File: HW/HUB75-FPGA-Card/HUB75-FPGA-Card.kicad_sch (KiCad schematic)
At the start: 4 parts

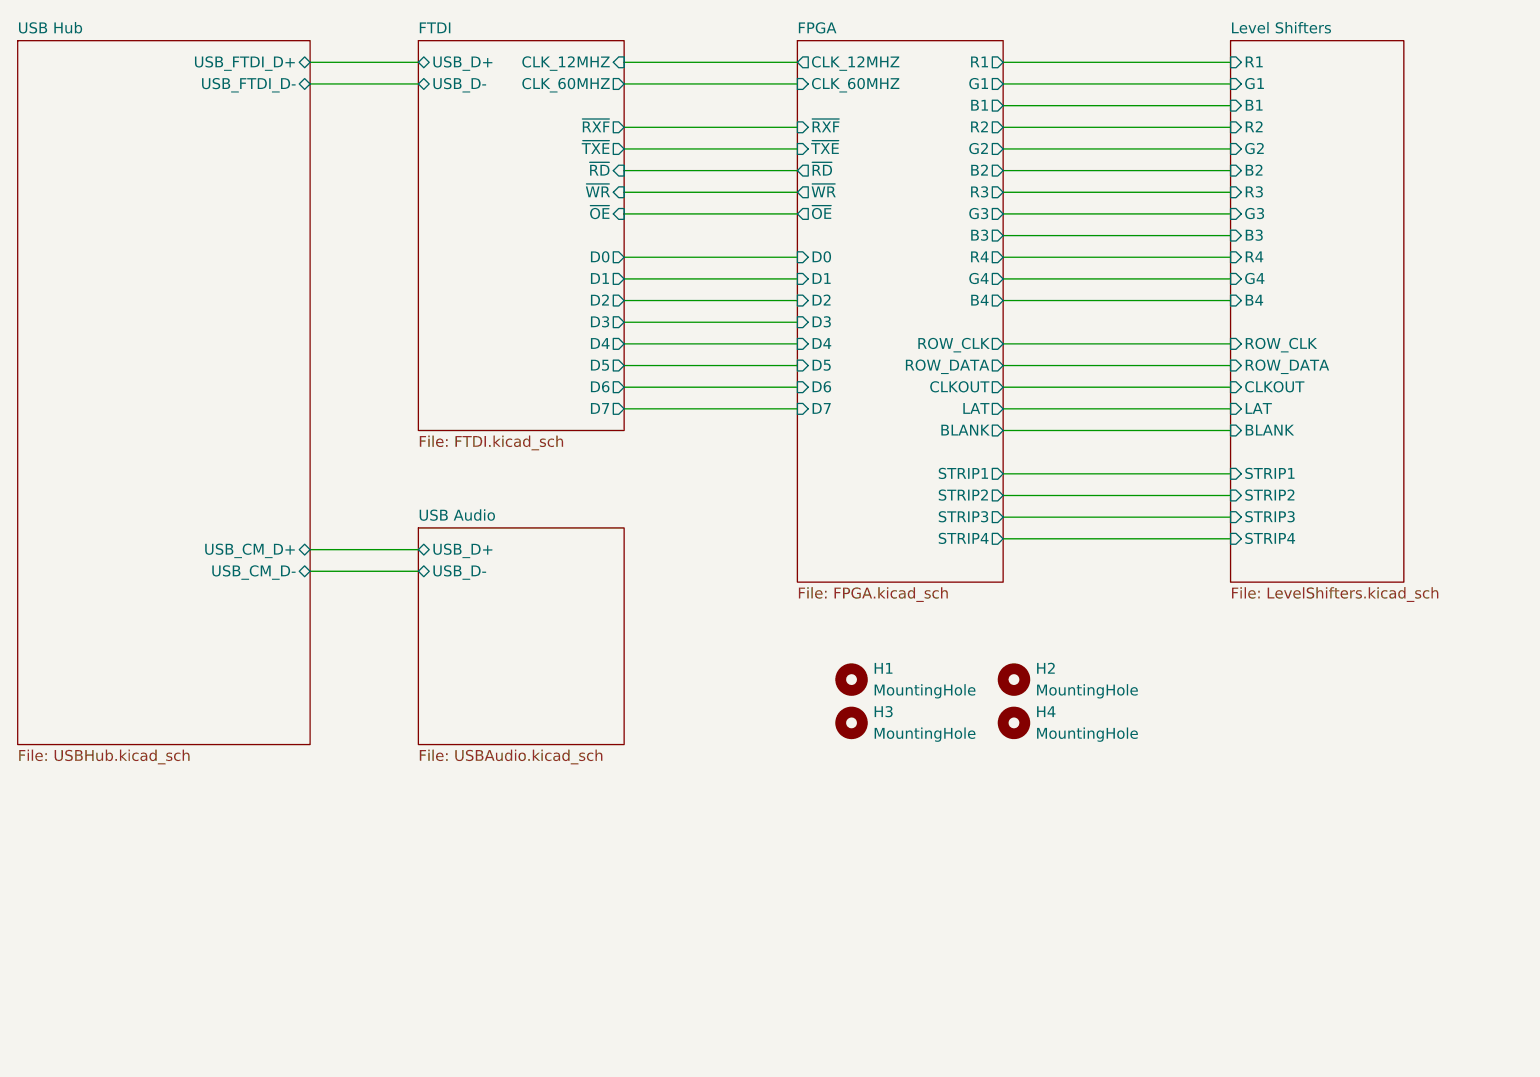
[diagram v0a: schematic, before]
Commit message: saving hardware progress
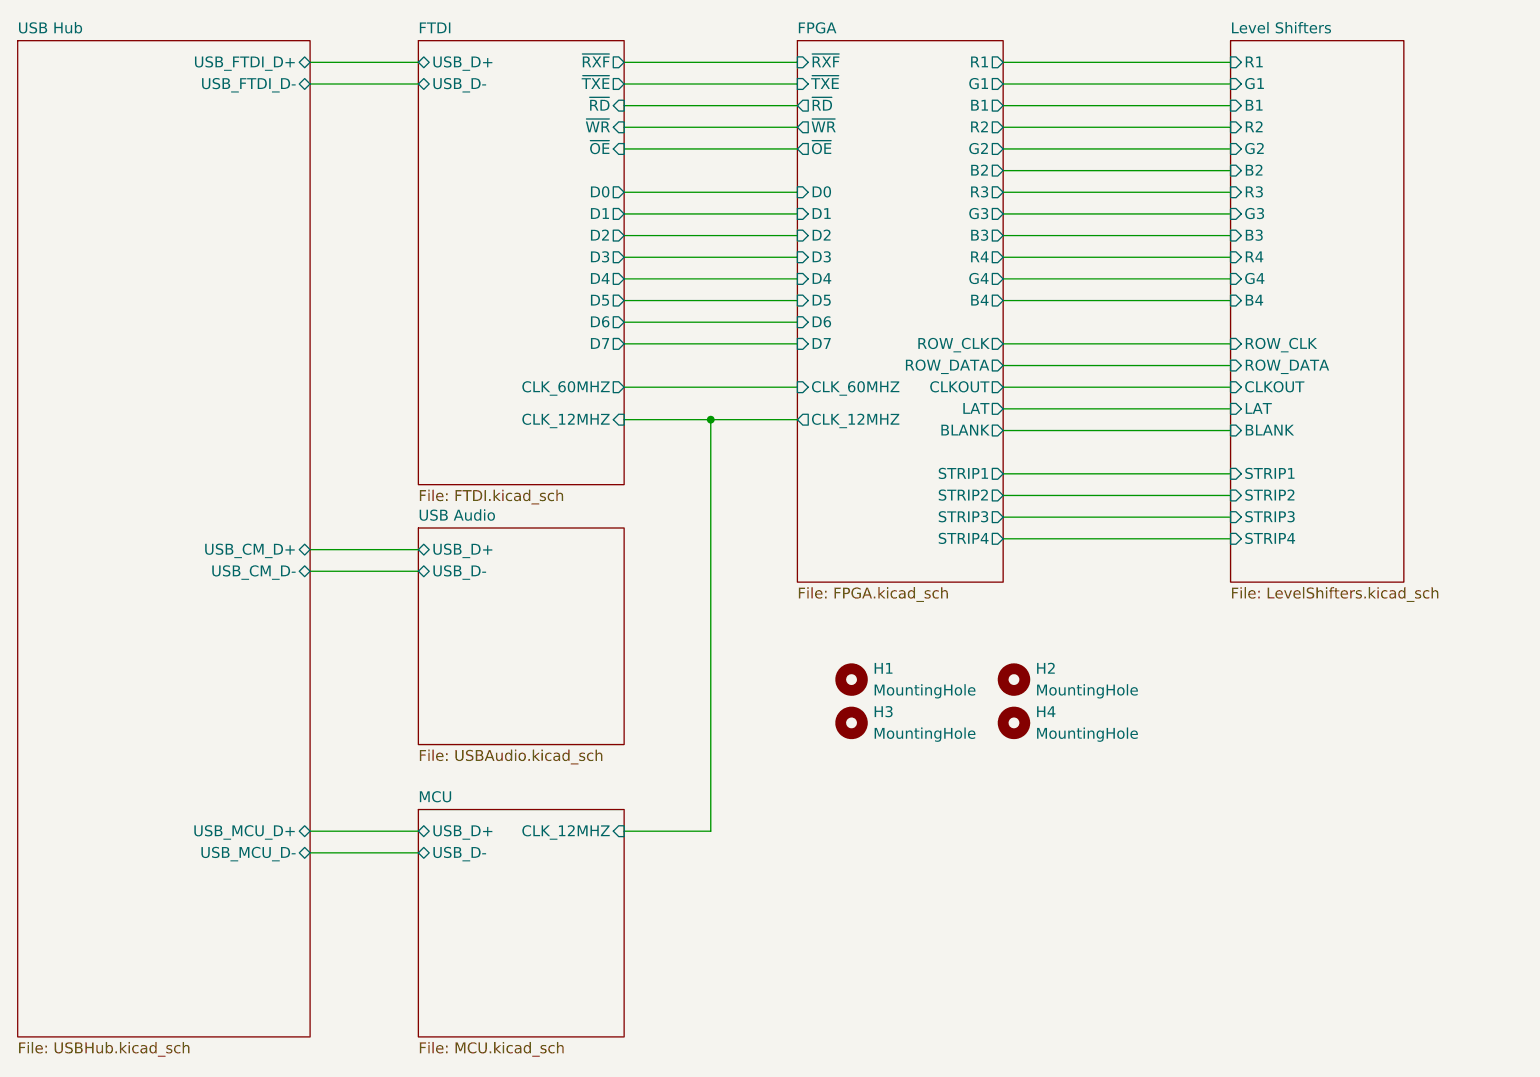
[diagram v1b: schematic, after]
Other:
- added sheet MCU (MCU.kicad_sch)
- sheet USB Hub ports: added USB_MCU_D+, USB_MCU_D-; removed none
